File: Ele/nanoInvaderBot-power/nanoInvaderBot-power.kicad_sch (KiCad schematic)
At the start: 31 parts, among them J1 S6B-ZR-SM4A-TF(LF)(SN), J2 S6B-ZR-SM4A-TF(LF)(SN), J3 1746142-1, J4 Conn_01x20, SW1 SW_SPDT, U4 BQ25170DSGR, U5 TLV61048DBVT

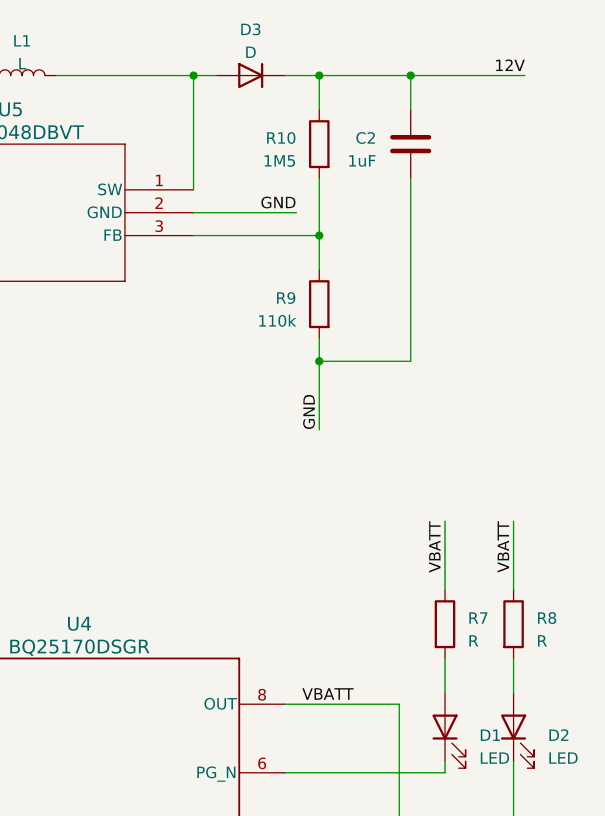
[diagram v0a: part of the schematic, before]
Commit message: Modifications for first running proto
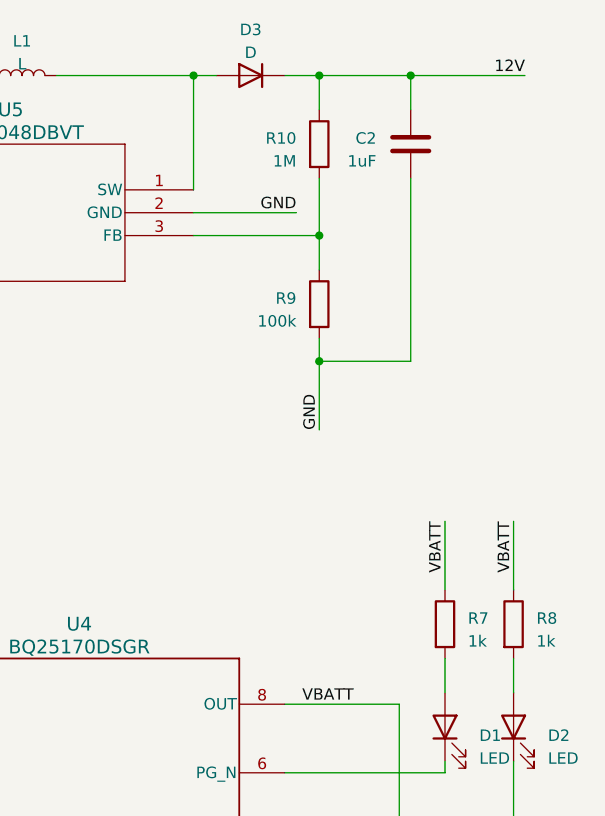
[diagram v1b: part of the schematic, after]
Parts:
- R10: value 1M5 -> 1M
- R7, R8: value R -> 1k
- R9: value 110k -> 100k
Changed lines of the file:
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@@
     )
   )
-  (symbol (lib_id "Device:R") (at 246.38 48.26 0) (mirror y) (unit 1)
-    (in_bom yes) (on_board yes) (dnp no) (fields_autoplaced)
+  (symbol (lib_id "Device:R") (at 246.38 48.26 0) (unit 1)
+    (in_bom yes) (on_board yes) (dnp no)
     (property "Reference" "R9" (at 243.84 47.625 0)
-      (effects (font (size 1.27 1.27)) (justify left))
-    )
-    (property "Value" "110k" (at 243.84 50.165 0)
-      (effects (font (size 1.27 1.27)) (justify left))
-    )
-    (property "Footprint" "Resistor_SMD:R_0402_1005Metric" (at 248.158 48.26 90)
+      (effects (font (size 1.27 1.27)) (justify right))
+    )
+    (property "Value" "100k" (at 243.84 50.165 0)
+      (effects (font (size 1.27 1.27)) (justify right))
+    )
+    (property "Footprint" "Resistor_SMD:R_0402_1005Metric" (at 244.602 48.26 90)
       (effects (font (size 1.27 1.27)) hide)
     )
@@
       (effects (font (size 1.27 1.27)) (justify left))
     )
-    (property "Value" "R" (at 262.89 85.725 0)
+    (property "Value" "1k" (at 262.89 85.725 0)
       (effects (font (size 1.27 1.27)) (justify left))
     )
@@
       (effects (font (size 1.27 1.27)) (justify left))
     )
-    (property "Value" "R" (at 270.51 85.725 0)
+    (property "Value" "1k" (at 270.51 85.725 0)
       (effects (font (size 1.27 1.27)) (justify left))
     )
@@
     )
   )
-  (symbol (lib_id "Device:R") (at 246.38 30.48 0) (mirror y) (unit 1)
-    (in_bom yes) (on_board yes) (dnp no) (fields_autoplaced)
+  (symbol (lib_id "Device:R") (at 246.38 30.48 0) (unit 1)
+    (in_bom yes) (on_board yes) (dnp no)
     (property "Reference" "R10" (at 243.84 29.845 0)
-      (effects (font (size 1.27 1.27)) (justify left))
-    )
-    (property "Value" "1M5" (at 243.84 32.385 0)
-      (effects (font (size 1.27 1.27)) (justify left))
-    )
-    (property "Footprint" "Resistor_SMD:R_0402_1005Metric" (at 248.158 30.48 90)
-      (effects (font (size 1.27 1.27)) hide)
-    )
+      (effects (font (size 1.27 1.27)) (justify right))
+    )
+    (property "Value" "1M" (at 243.84 32.385 0)
+      (effects (font (size 1.27 1.27)) (justify right))
+    )
+    (property "Footprint" "Resistor_SMD:R_0402_1005Metric" (at 244.602 30.48 90)
+      (effects (font (size 1.27 1.27)) hide)
+    )
